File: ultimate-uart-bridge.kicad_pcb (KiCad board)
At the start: 2 copper layers, 20 parts, among them J101 USB_B_Micro, J102 Conn_01x03, J103 Conn_01x03

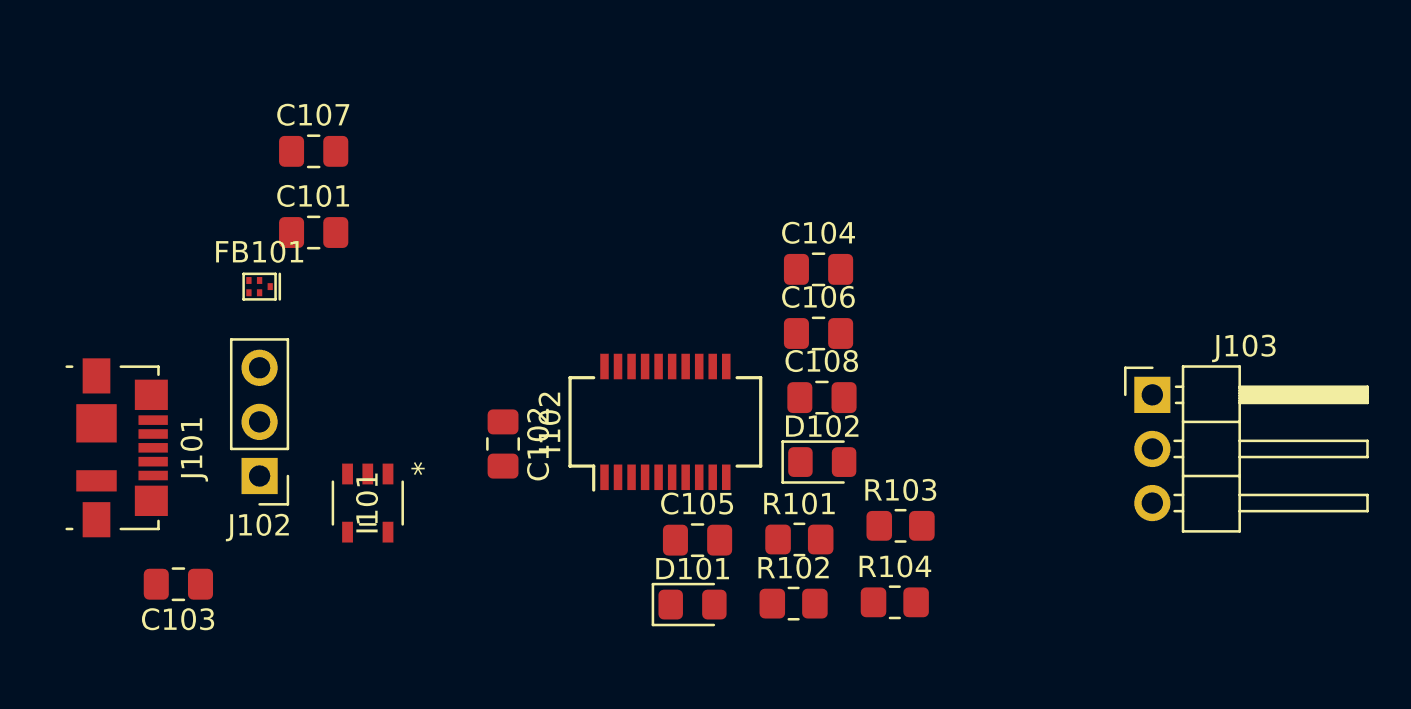
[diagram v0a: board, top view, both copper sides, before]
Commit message: First Routing
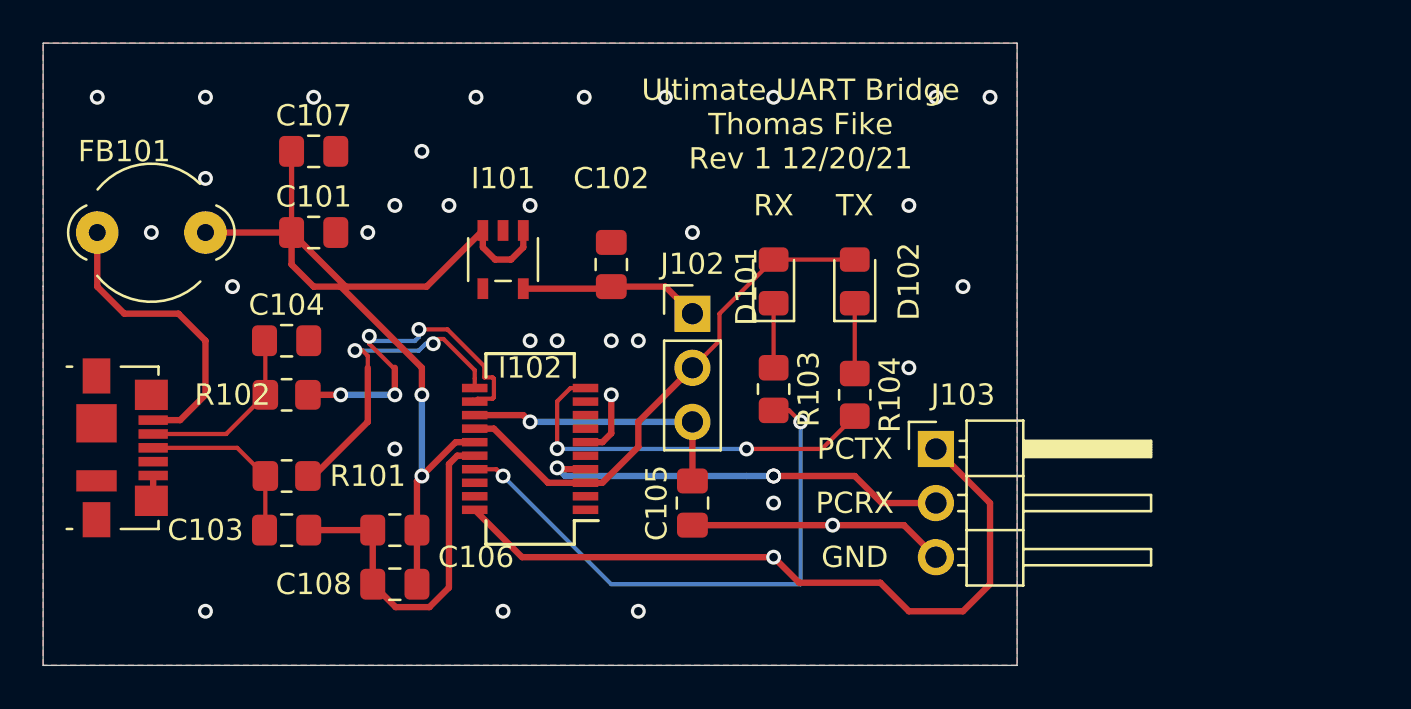
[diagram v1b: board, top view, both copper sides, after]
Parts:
- FB101: footprint Filter:Filter_1411-5_1.4x1.1mm -> Ferrite_THT:LairdTech_28C0236-0JW-10
- moved R102 25.7 mm to (113.0, 90.2)
- moved C104 25.2 mm to (113.0, 87.6)
- moved R101 24.3 mm to (113.0, 94.0)
- moved C106 21.9 mm to (118.1, 96.5), turned to 180 degrees
- moved C108 21.9 mm to (118.1, 99.1), turned to 180 degrees
- moved J102 21.7 mm to (132.1, 86.4), turned to 0 degrees
- moved D101 15.6 mm to (135.9, 84.8), turned to 90 degrees
- moved I101 13.1 mm to (123.2, 83.8)
- moved J103 10.5 mm to (143.5, 92.7)
- moved R104 9.92 mm to (139.7, 90.2), turned to 270 degrees
- moved C102 9.84 mm to (128.3, 84.1), turned to 90 degrees
- moved R103 8.76 mm to (135.9, 89.9), turned to 270 degrees
- moved D102 8.62 mm to (139.7, 84.8), turned to 90 degrees
- moved I102 6.48 mm to (124.5, 92.7), turned to 180 degrees
- moved C103 5.68 mm to (113.0, 96.5), turned to 0 degrees
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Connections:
- net USB_DM renamed USBD_N
- net USB_DP renamed USBD_P
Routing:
- net VBUS: track 0.00 -> 46.0 mm, vias 0 -> 2
- net /PCTX: track 0.00 -> 34.1 mm, vias 0 -> 1
- net GND: track 0.00 -> 33.6 mm, vias 0 -> 32
- net /RXLED#: track 0.00 -> 26.6 mm, vias 0 -> 2
- net VCCIO: track 0.00 -> 24.7 mm
- net /PCRX: track 0.00 -> 19.8 mm, vias 0 -> 3
- net /TXLED#: track 0.00 -> 18.4 mm, vias 0 -> 2
- net USBD_N: track 0.00 -> 17.0 mm, vias 0 -> 4
- net USBD_P: track 0.00 -> 15.1 mm, vias 0 -> 2
- net Net-(FB101-Pad2): track 0.00 -> 14.2 mm
- net +3V3: track 0.00 -> 13.1 mm, vias 0 -> 1
- net Net-(C104-Pad1): track 0.00 -> 8.58 mm
- net +1V8: track 0.00 -> 8.51 mm
- net Net-(C103-Pad1): track 0.00 -> 8.37 mm
- net Net-(D102-Pad1): track 0.00 -> 3.30 mm
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- added copper zone on B.Cu, net GND
- added copper zone on F.Cu, net GND
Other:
- board outline added: 45.7 x 29.2 mm
- net class Default: trace_width 0.25 -> 0.2; via_dia 0.8 -> 0.7
- rule trace_min: 0.2 -> 0.128
- rule via_min_size: 0.4 -> 0.6
- board text added: "GND"
- board text added: "JLCJLCJLCJLC"
- board text added: "PCRX"
- board text added: "PCTX"
- board text added: "RX"
- board text added: "TX"
- board text added: "Ultimate UART Bridge Thomas Fike Rev 1 12/20/21"

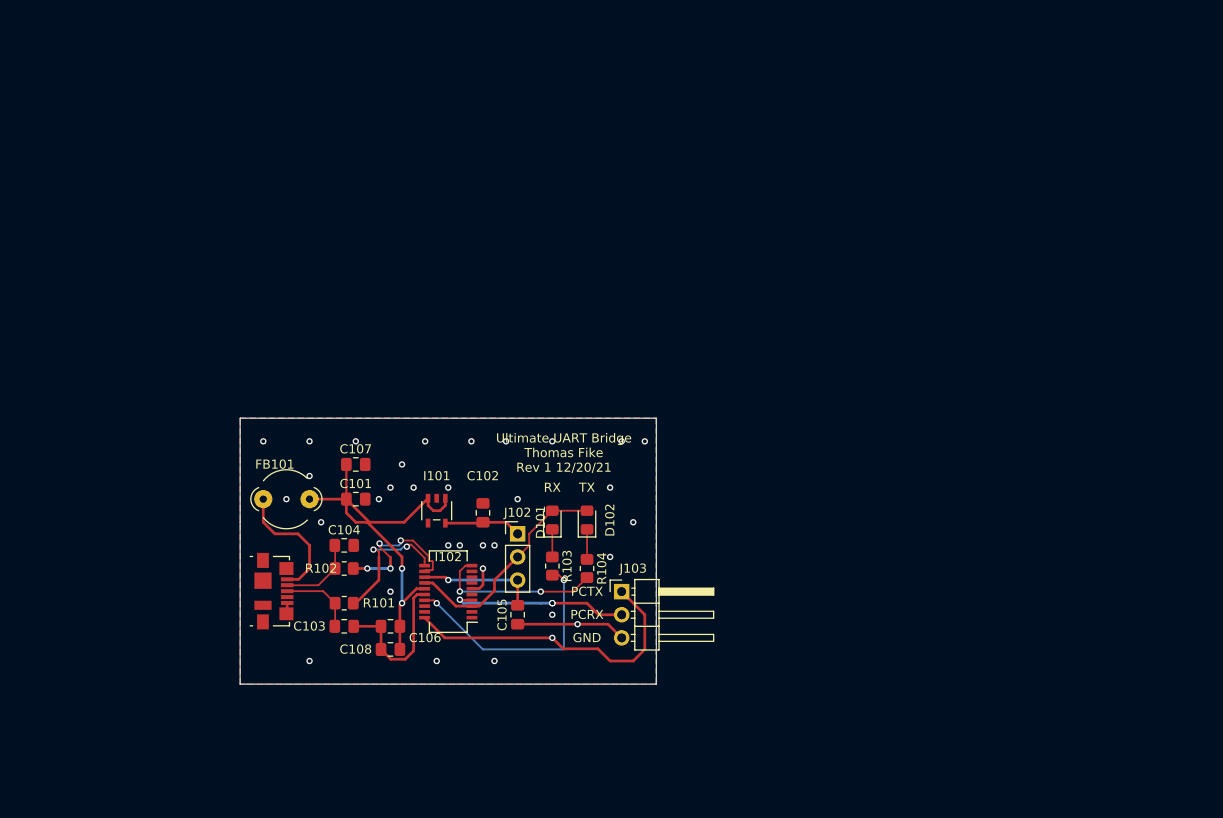
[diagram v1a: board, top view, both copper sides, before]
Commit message: New inital routing
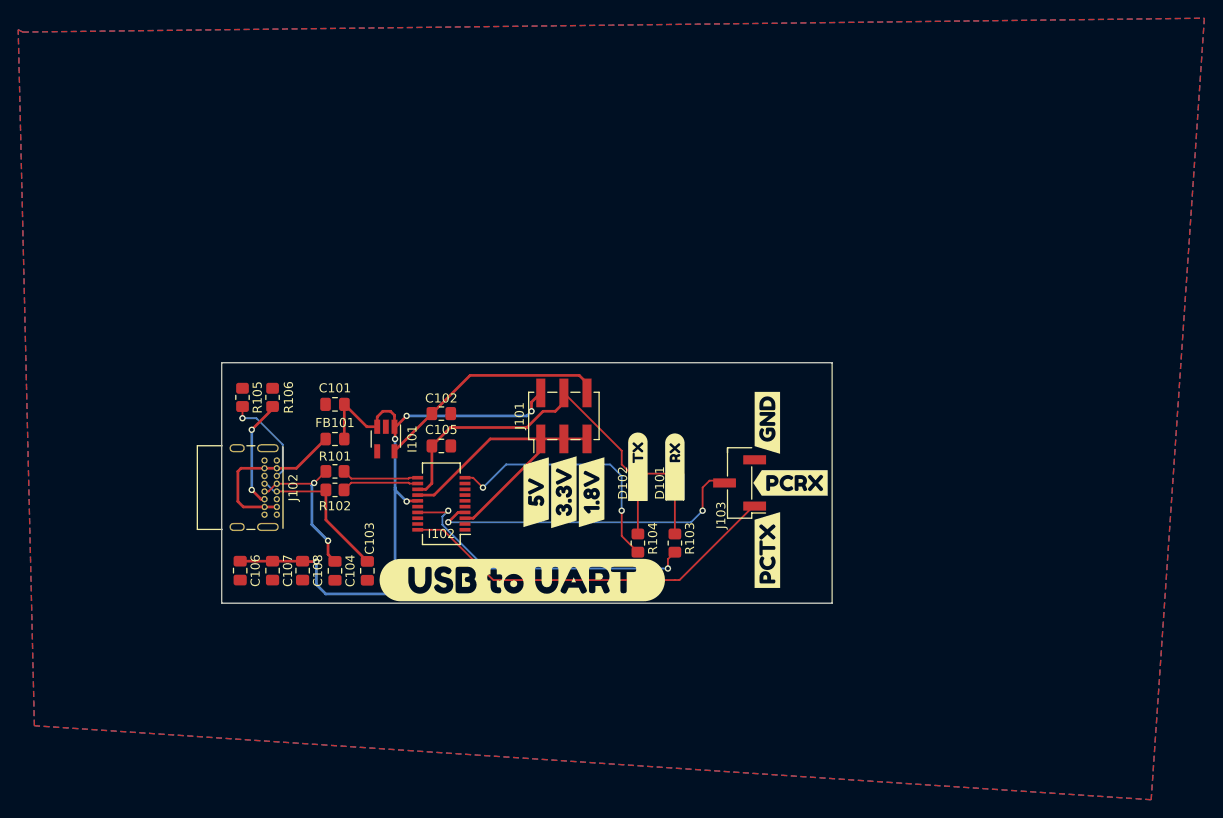
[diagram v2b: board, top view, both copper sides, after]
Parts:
- added R105: 5.1k, Resistor_SMD:R_0805_2012Metric_Pad1.20x1.40mm_HandSolder, F.Cu at (101.9, 71.4)
- added R106: 5.1k, Resistor_SMD:R_0805_2012Metric_Pad1.20x1.40mm_HandSolder, F.Cu at (105.2, 71.4)
- added kibuzzard-62CBA051: G***, kibuzzard-62CBA051, F.Cu at (159.5, 74.2)
- added kibuzzard-62CBA0C9: G***, kibuzzard-62CBA0C9, F.Cu at (159.5, 88.1)
- added kibuzzard-62CBA130: G***, kibuzzard-62CBA130, F.Cu at (162.1, 80.8)
- added kibuzzard-62CBA316: G***, kibuzzard-62CBA316, F.Cu at (149.4, 79.0)
- added kibuzzard-62CBA331: G***, kibuzzard-62CBA331, F.Cu at (145.3, 79.0)
- added kibuzzard-62CBA409: G***, kibuzzard-62CBA409, F.Cu at (140.2, 81.8)
- added kibuzzard-62CBA40F: G***, kibuzzard-62CBA40F, F.Cu at (137.2, 81.8)
- added kibuzzard-62CBA429: G***, kibuzzard-62CBA429, F.Cu at (134.1, 81.8)
- added kibuzzard-62CBA9F2: G***, kibuzzard-62CBA9F2, F.Cu at (132.6, 91.4)
- FB101: footprint Ferrite_THT:LairdTech_28C0236-0JW-10 -> Inductor_SMD:L_0805_2012Metric_Pad1.15x1.40mm_HandSolder
- I101: footprint footprints:MIC5317-1.8YM5-TR -> Package_TO_SOT_SMD:SOT-23-5_HandSoldering
- J101: value USB_B_Micro -> Conn_02x03_Row_Letter_First; footprint Connector_USB:USB_Micro-B_Molex_47346-0001 -> Connector_PinHeader_2.54mm:PinHeader_2x03_P2.54mm_Vertical_SMD
- J102: value Conn_01x03 -> USB_C_Receptacle_USB2.0; footprint Connector_PinHeader_2.54mm:PinHeader_1x03_P2.54mm_Vertical -> Connector_USB:USB_C_Receptacle_GCT_USB4085
- J103: footprint Connector_PinHeader_2.54mm:PinHeader_1x03_P2.54mm_Horizontal -> Connector_PinHeader_2.54mm:PinHeader_1x03_P2.54mm_Vertical_SMD_Pin1Left
- moved J101 37.2 mm to (137.2, 73.4), turned to 90 degrees
- moved J102 27.7 mm to (105.6, 78.3), turned to -90 degrees
- moved C105 20.3 mm to (123.7, 76.7), turned to 180 degrees
- moved J103 17.6 mm to (156.5, 80.8), turned to 180 degrees
- moved C106 17.6 mm to (101.6, 90.4), turned to -90 degrees
- moved C107 14.8 mm to (105.2, 90.4), turned to -90 degrees
- moved R101 14.5 mm to (112.0, 79.5)
- moved D101 14.1 mm to (149.4, 80.8)
- moved R103 13.7 mm to (149.4, 87.4)
- moved C108 13.0 mm to (108.5, 90.4), turned to -90 degrees
- moved C102 11.8 mm to (123.7, 73.2), turned to 0 degrees
- moved C101 10.7 mm to (112.0, 72.1), turned to 180 degrees
- moved I102 9.68 mm to (123.7, 83.1)
- moved I101 9.66 mm to (117.6, 75.9)
- moved R102 8.70 mm to (112.0, 81.5)
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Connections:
- D101 pad 2: VCCIO -> +3V3
- D102 pad 2: VCCIO -> +3V3
- I101 pad 4: Net-(I101-Pad4) -> unconnected-(I101-Pad4)
- I102 pad 1: Net-(I102-Pad1) -> unconnected-(I102-Pad1)
- I102 pad 18: Net-(I102-Pad18) -> unconnected-(I102-Pad18)
- I102 pad 19: Net-(I102-Pad19) -> unconnected-(I102-Pad19)
- I102 pad 2: Net-(I102-Pad2) -> unconnected-(I102-Pad2)
- I102 pad 5: Net-(I102-Pad5) -> unconnected-(I102-Pad5)
- I102 pad 7: Net-(I102-Pad7) -> unconnected-(I102-Pad7)
- I102 pad 8: Net-(I102-Pad8) -> unconnected-(I102-Pad8)
- I102 pad 9: Net-(I102-Pad9) -> unconnected-(I102-Pad9)
- J101 pad 1: Net-(FB101-Pad2) -> VCCIO
- J101 pad 2: Net-(C104-Pad1) -> VBUS
- J101 pad 3: Net-(C103-Pad1) -> VCCIO
- J101 pad 4: Net-(J101-Pad4) -> +3V3
- J101 pad 5: GND -> VCCIO
- J101 pad 6: GND -> +1V8
- R101 pad 1: Net-(C103-Pad1) -> Net-(C104-Pad1)
- R102 pad 1: Net-(C104-Pad1) -> Net-(C103-Pad1)
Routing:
- net GND: track 33.6 -> 0.00 mm, vias 32 -> 0
- net +3V3: track 13.1 -> 40.2 mm, vias 1 -> 0
- net VBUS: track 46.0 -> 73.0 mm, vias 2 -> 5
- net +1V8: track 8.51 -> 26.1 mm
- net /PCRX: track 19.8 -> 36.1 mm, vias 3 -> 2
- net Net-(J102-PadB5): track 0.00 -> 11.9 mm, vias 0 -> 2
- net Net-(J102-PadA5): track 0.00 -> 10.7 mm, vias 0 -> 1
- net /TXLED#: track 18.4 -> 28.3 mm
- net VCCIO: track 24.7 -> 33.8 mm
- net Net-(C104-Pad1): track 8.58 -> 17.5 mm, vias 0 -> 2
- net USBD_N: track 17.0 -> 8.45 mm, vias 4 -> 0
- net Net-(C103-Pad1): track 8.37 -> 16.9 mm
- net /PCTX: track 34.1 -> 42.5 mm, vias 1 -> 0
- net /RXLED#: track 26.6 -> 34.1 mm
- net USBD_P: track 15.1 -> 8.45 mm, vias 2 -> 0
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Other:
- board size 45.7 x 29.2 mm -> 67.1 x 26.4 mm
- net class Default removed
- board text removed: "GND"
- board text removed: "JLCJLCJLCJLC"
- board text removed: "PCRX"
- board text removed: "PCTX"
- board text removed: "RX"
- board text removed: "TX"
- board text removed: "Ultimate UART Bridge Thomas Fike Rev 1 12/20/21"
